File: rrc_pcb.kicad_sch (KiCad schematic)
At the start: 15 parts, among them J1 Conn_01x02_Male-Connector, J2 Conn_01x03_Male-Connector, J3 digital logic connection, U1 iridium9602, U2 Teensy4.1, U3 BN220-GPS, U4 ICM-20948, U5 MS5611, U6 logo, U7 voltReg

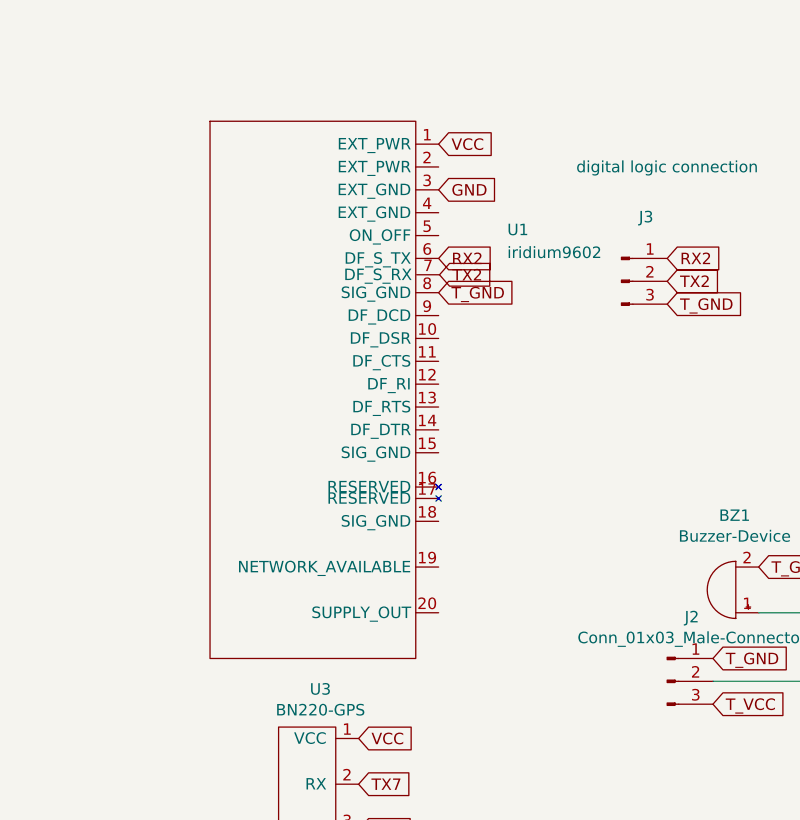
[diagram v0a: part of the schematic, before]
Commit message: rfd iteration f3
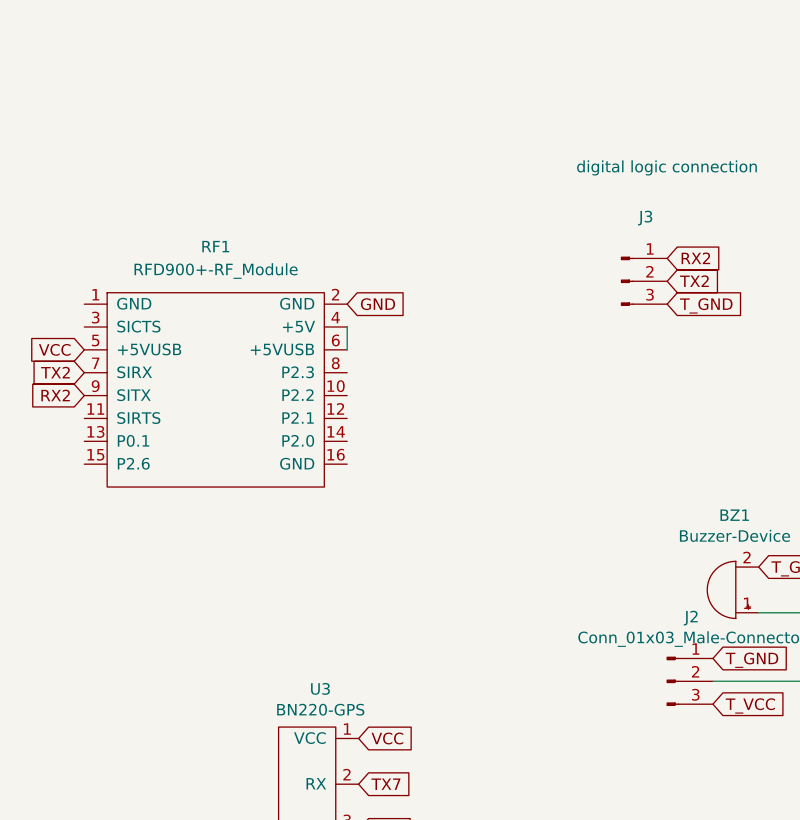
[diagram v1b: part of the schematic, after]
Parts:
- removed U1: iridium9602, iridium9602:iridium9602, symbol parts:iridium9602
- added RF1: RFD900+-RF_Module, rfd900+:RFD900+, symbol parts:RFD900+-RF_Module
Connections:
- net GND: now also RF1.2 (GND)
- net RX2: now also RF1.9 (SITX)
- net TX2: now also RF1.7 (SIRX)
- net VCC: now also RF1.5 (+5VUSB)
- new net: RF1.4 (+5V), RF1.6 (+5VUSB)
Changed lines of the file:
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@@
 (kicad_sch (version 20211123) (generator eeschema)
   (paper "A4")
+  (wire (pts (xy 36.83 35.56) (xy 36.83 38.1))
+    (stroke (width 0) (type default) (color 0 0 0 0))
+  )
   (wire (pts (xy 241.3 105.41) (xy 229.87 105.41))
     (stroke (width 0) (type default) (color 0 0 0 0))
@@
     )
   )
-  (global_label "TX2" (shape input) (at 47.0887 29.7566 0) (fields_autoplaced)
-    (effects (font (size 1.27 1.27)) (justify left))
-    (property "Intersheet References" "${INTERSHEET_REFS}" (id 0) (at 52.7996 29.6772 0)
-      (effects (font (size 1.27 1.27)) (justify left) hide)
+  (global_label "TX2" (shape input) (at 7.62 40.64 180) (fields_autoplaced)
+    (effects (font (size 1.27 1.27)) (justify right))
+    (property "Intersheet References" "${INTERSHEET_REFS}" (id 0) (at 1.9091 40.7194 0)
+      (effects (font (size 1.27 1.27)) (justify right) hide)
     )
   )
@@
     )
   )
-  (global_label "VCC" (shape input) (at 46.99 15.24 0) (fields_autoplaced)
-    (effects (font (size 1.27 1.27)) (justify left))
-    (property "Intersheet References" "${INTERSHEET_REFS}" (id 0) (at -121.92 -113.03 0)
+  (global_label "VCC" (shape input) (at 7.62 38.1 180) (fields_autoplaced)
+    (effects (font (size 1.27 1.27)) (justify right))
+    (property "Intersheet References" "${INTERSHEET_REFS}" (id 0) (at 176.53 166.37 0)
       (effects (font (size 1.27 1.27)) hide)
     )
@@
     )
   )
-  (global_label "RX2" (shape input) (at 46.99 27.94 0) (fields_autoplaced)
-    (effects (font (size 1.27 1.27)) (justify left))
-    (property "Intersheet References" "${INTERSHEET_REFS}" (id 0) (at 53.0032 27.8606 0)
-      (effects (font (size 1.27 1.27)) (justify left) hide)
+  (global_label "RX2" (shape input) (at 7.62 43.18 180) (fields_autoplaced)
+    (effects (font (size 1.27 1.27)) (justify right))
+    (property "Intersheet References" "${INTERSHEET_REFS}" (id 0) (at 1.6068 43.2594 0)
+      (effects (font (size 1.27 1.27)) (justify right) hide)
     )
   )
@@
     )
   )
-  (global_label "T_GND" (shape input) (at 46.99 31.75 0) (fields_autoplaced)
-    (effects (font (size 1.27 1.27)) (justify left))
-    (property "Intersheet References" "${INTERSHEET_REFS}" (id 0) (at -19.05 -13.97 0)
-      (effects (font (size 1.27 1.27)) hide)
-    )
-  )
   (global_label "T_GND" (shape input) (at 38.1 95.25 0) (fields_autoplaced)
     (effects (font (size 1.27 1.27)) (justify left))
@@
     )
   )
-  (global_label "GND" (shape input) (at 46.99 20.32 0) (fields_autoplaced)
-    (effects (font (size 1.27 1.27)) (justify left))
-    (property "Intersheet References" "${INTERSHEET_REFS}" (id 0) (at -25.4 -81.28 0)
+  (global_label "GND" (shape input) (at 36.83 33.02 0) (fields_autoplaced)
+    (effects (font (size 1.27 1.27)) (justify left))
+    (property "Intersheet References" "${INTERSHEET_REFS}" (id 0) (at -35.56 -68.58 0)
       (effects (font (size 1.27 1.27)) hide)
     )
@@
     (pin "9")
   )
-  (symbol (lib_id "parts:iridium9602") (at 34.29 21.59 0) (unit 1)
+  (symbol (lib_id "rrc_pcb-rescue:Conn_01x03_Male-Connector") (at 67.31 30.48 0) (unit 1)
+    (in_bom yes) (on_board yes)
+    (property "Reference" "J3" (id 0) (at 70.0532 23.3426 0))
+    (property "Value" "digital logic connection" (id 1) (at 72.39 17.78 0))
+    (property "Footprint" "Connector_PinHeader_2.54mm:PinHeader_1x03_P2.54mm_Vertical" (id 2) (at 67.31 30.48 0)
+      (effects (font (size 1.27 1.27)) hide)
+    )
+    (property "Datasheet" "~" (id 3) (at 67.31 30.48 0)
+      (effects (font (size 1.27 1.27)) hide)
+    )
+    (pin "1")
+    (pin "2")
+    (pin "3")
+  )
+  (symbol (lib_id "parts:RFD900+-RF_Module") (at 13.97 33.02 0) (unit 1)
     (in_bom yes) (on_board yes) (fields_autoplaced)
-    (property "Reference" "U1" (id 0) (at 54.61 24.7649 0)
-      (effects (font (size 1.27 1.27)) (justify left))
-    )
-    (property "Value" "iridium9602" (id 1) (at 54.61 27.3049 0)
-      (effects (font (size 1.27 1.27)) (justify left))
-    )
-    (property "Footprint" "iridium9602:iridium9602" (id 2) (at 34.29 21.59 0)
-      (effects (font (size 1.27 1.27)) hide)
-    )
-    (property "Datasheet" "" (id 3) (at 34.29 21.59 0)
+    (property "Reference" "RF1" (id 0) (at 22.225 26.67 0))
+    (property "Value" "RFD900+-RF_Module" (id 1) (at 22.225 29.21 0))
+    (property "Footprint" "rfd900+:RFD900+" (id 2) (at 13.97 33.02 0)
+      (effects (font (size 1.27 1.27)) hide)
+    )
+    (property "Datasheet" "" (id 3) (at 13.97 33.02 0)
       (effects (font (size 1.27 1.27)) hide)
     )
@@
     (pin "15")
     (pin "16")
-    (pin "17")
-    (pin "18")
-    (pin "19")
-    (pin "2")
-    (pin "20")
+    (pin "2")
     (pin "3")
     (pin "4")
@@
     (pin "8")
     (pin "9")
-  )
-  (symbol (lib_id "rrc_pcb-rescue:Conn_01x03_Male-Connector") (at 67.31 30.48 0) (unit 1)
-    (in_bom yes) (on_board yes)
-    (property "Reference" "J3" (id 0) (at 70.0532 23.3426 0))
-    (property "Value" "digital logic connection" (id 1) (at 72.39 17.78 0))
-    (property "Footprint" "Connector_PinHeader_2.54mm:PinHeader_1x03_P2.54mm_Vertical" (id 2) (at 67.31 30.48 0)
-      (effects (font (size 1.27 1.27)) hide)
-    )
-    (property "Datasheet" "~" (id 3) (at 67.31 30.48 0)
-      (effects (font (size 1.27 1.27)) hide)
-    )
-    (pin "1")
-    (pin "2")
-    (pin "3")
   )
   (symbol (lib_id "teensy:Teensy4.1") (at 127 76.2 0) (unit 1)
@@
       (reference "R4") (unit 1) (value "R-Device") (footprint "Resistor_THT:R_Axial_DIN0207_L6.3mm_D2.5mm_P10.16mm_Horizontal")
     )
-    (path "/84f80ca1-29d4-4e34-8c20-e0b5bcec9cb7"
-      (reference "U1") (unit 1) (value "iridium9602") (footprint "iridium9602:iridium9602")
+    (path "/cca84f39-62d3-48b7-ab11-081e484cf270"
+      (reference "RF1") (unit 1) (value "RFD900+-RF_Module") (footprint "rfd900+:RFD900+")
     )
     (path "/e2a4979b-162a-4acf-966e-29cd5e9f5e0d"
